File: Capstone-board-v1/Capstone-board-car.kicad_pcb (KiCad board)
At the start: 2 copper layers, 54.3 x 54.3 mm, 25 parts, among them J1 Pico Socket 1, J2 Pico Socket 2, J3 Ultra Sonic Sensor, J4 Car, J5 Camera, J6 Gyroscope Sensor, U1 3.3V V.R, U2 555 Timer, U3 5V V.R 2, U4 5V V.R 1

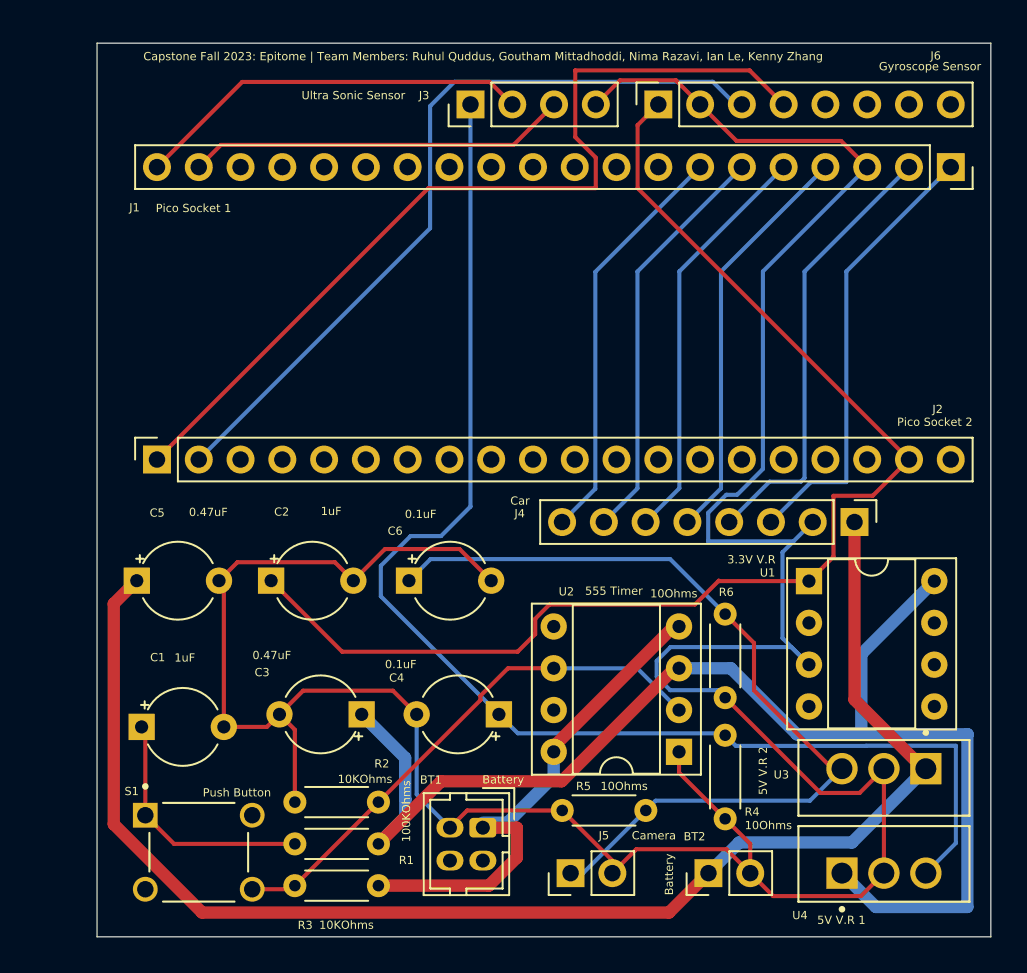
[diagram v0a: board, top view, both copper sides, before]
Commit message: Final PCBs done!
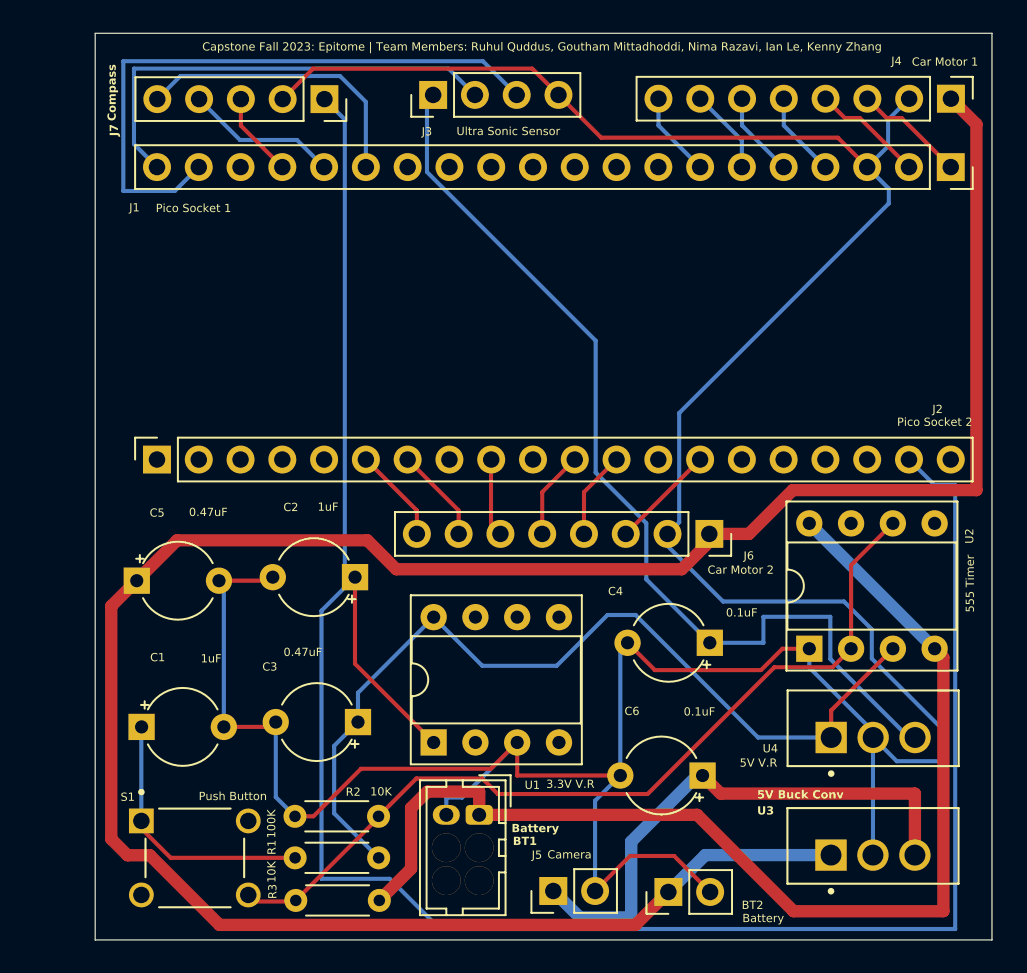
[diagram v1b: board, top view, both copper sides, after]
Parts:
- removed R4, R5, R6: 10Ohms, Resistor_THT:R_Axial_DIN0204_L3.6mm_D1.6mm_P5.08mm_Horizontal
- added J7: Compass, Connector_PinSocket_2.54mm:PinSocket_1x05_P2.54mm_Vertical, F.Cu at (49.5, 73.8)
- BT1: footprint Connector_Hirose:Hirose_DF11-4DP-2DSA_2x02_P2.00mm_Vertical -> Connector_Hirose:Hirose_DF11-6DP-2DSA_2x03_P2.00mm_Vertical
- J4: value Car -> Car Motor 1
- J6: value Gyroscope Sensor -> Car Motor 2
- R1: value 100KOhms -> 100K
- R2, R3: value 10KOhms -> 10K
- U3: value 5V V.R 2 -> 5V Buck Conv
- U4: value 5V V.R 1 -> 5V V.R
- moved J4 26.4 mm to (87.6, 73.8)
- moved J6 26.3 mm to (73.0, 100.3), turned to -90 degrees
- moved U1 24.8 mm to (56.2, 113.0), turned to 90 degrees
- moved C6 21.4 mm to (72.5, 115.0), turned to 180 degrees
- moved C4 13.5 mm to (73.0, 106.9)
- moved U2 10.1 mm to (79.0, 107.3), turned to 90 degrees
- moved U4 8.27 mm to (80.4, 112.7)
- moved U3 7.80 mm to (80.3, 119.8), turned to 0 degrees
- moved C2 5.11 mm to (51.4, 102.9), turned to 180 degrees
- moved BT2 2.69 mm to (70.5, 122.0)
- moved J3 2.34 mm to (56.2, 73.6)
- moved J5 1.51 mm to (63.5, 122.0)
- moved R3 0.90 mm to (47.8, 122.6)
- moved R2 0.86 mm to (47.8, 117.5)
- moved R1 0.85 mm to (47.8, 120.0)
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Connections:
- J1 pad 15: unconnected-(J1-Pin_15-Pad15) -> Net-(J1-Pin_15)
- J1 pad 16: unconnected-(J1-Pin_16-Pad16) -> Net-(J1-Pin_16)
- J1 pad 17: unconnected-(J1-Pin_17-Pad17) -> Net-(J1-Pin_17)
- J2 pad 1: Net-(J2-Pin_1) -> unconnected-(J2-Pin_1-Pad1)
- J2 pad 11: unconnected-(J2-Pin_11-Pad11) -> Net-(J2-Pin_11)
- J2 pad 12: unconnected-(J2-Pin_12-Pad12) -> Net-(J2-Pin_12)
- J2 pad 14: unconnected-(J2-Pin_14-Pad14) -> Net-(J2-Pin_14)
- J2 pad 2: Net-(J2-Pin_2) -> unconnected-(J2-Pin_2-Pad2)
- J2 pad 6: unconnected-(J2-Pin_6-Pad6) -> Net-(J2-Pin_6)
- J2 pad 7: unconnected-(J2-Pin_7-Pad7) -> Net-(J2-Pin_7)
- J2 pad 9: unconnected-(J2-Pin_9-Pad9) -> Net-(J2-Pin_9)
- J6 pad 1: Net-(J2-Pin_19) -> VCCQ
- J6 pad 3: Net-(J2-Pin_2) -> Net-(J2-Pin_14)
- J6 pad 4: Net-(J2-Pin_1) -> Net-(J2-Pin_12)
- J6 pad 5: unconnected-(J6-Pin_5-Pad5) -> Net-(J2-Pin_11)
- J6 pad 6: unconnected-(J6-Pin_6-Pad6) -> Net-(J2-Pin_9)
- J6 pad 7: unconnected-(J6-Pin_7-Pad7) -> Net-(J2-Pin_7)
- J6 pad 8: unconnected-(J6-Pin_8-Pad8) -> Net-(J2-Pin_6)
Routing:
- net VCCQ: track 87.5 -> 144.8 mm
- net Net-(J2-Pin_1): track 54.7 -> 0.00 mm
- net Net-(J2-Pin_19): track 77.1 -> 131.3 mm
- net Net-(J2-Pin_2): track 47.5 -> 0.00 mm
- net VCC: track 31.2 -> 70.0 mm
- net Net-(U1-IN): track 82.8 -> 55.0 mm
- net Net-(J3-Pin_1): track 80.5 -> 59.2 mm
- net Net-(J1-Pin_1): track 27.4 -> 6.79 mm
- net Net-(J1-Pin_2): track 27.2 -> 6.79 mm
- net Net-(U2-THR): track 32.7 -> 52.6 mm
- net Net-(J1-Pin_6): track 25.1 -> 5.21 mm
- net Net-(J1-Pin_4): track 25.1 -> 5.21 mm
- net Net-(J1-Pin_7): track 25.1 -> 5.21 mm
- net Net-(J1-Pin_5): track 25.1 -> 5.21 mm
- net Net-(J5-Pin_1): track 53.0 -> 33.1 mm
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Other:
- board size 54.3 x 54.3 mm -> 54.5 x 55.1 mm
